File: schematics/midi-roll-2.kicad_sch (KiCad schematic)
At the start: 21 parts, among them M1 Stepper_Motor_unipolar_5pin, SW1 SW_Push_SPDT, SW10 SW_Push_SPDT, SW11 SW_Push_SPDT, SW12 SW_Push_SPDT, SW13 SW_Push_SPDT, SW14 SW_Push_SPDT, SW15 SW_Push_SPDT, SW16 SW_Push_SPDT, SW2 SW_Push_SPDT, SW3 SW_Push_SPDT, SW4 SW_Push_SPDT, SW5 SW_Push_SPDT, SW6 SW_Push_SPDT, SW7 SW_Push_SPDT, SW8 SW_Push_SPDT, SW9 SW_Push_SPDT, U1 WeMos_D1_mini, U2 CD4051B, U3 CD4051B, U4 ULN2003A

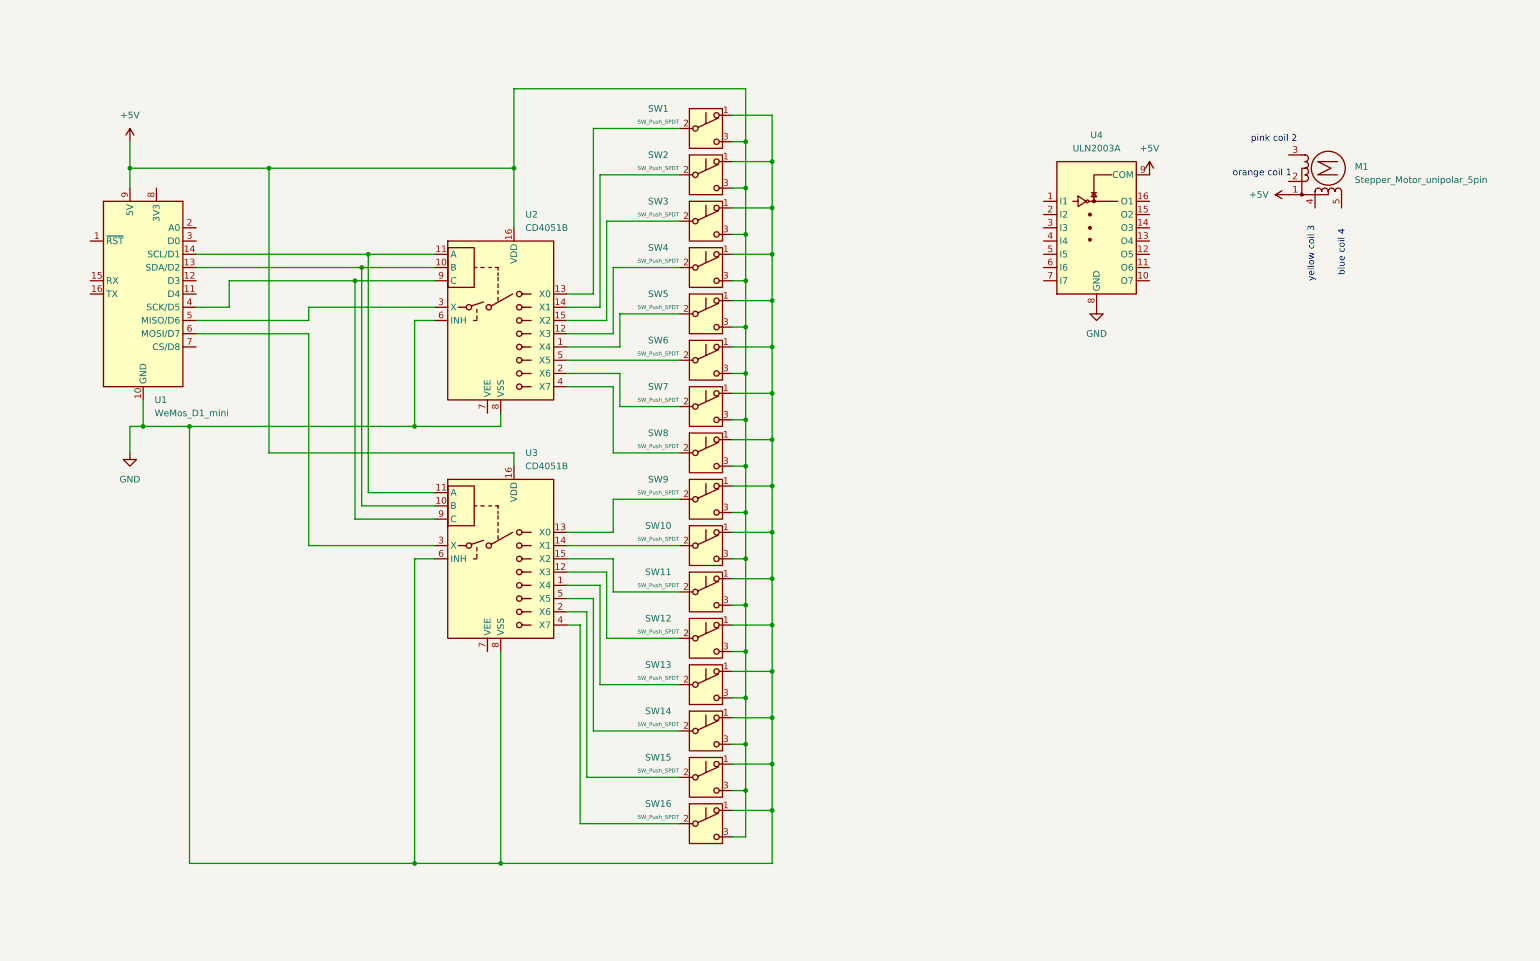
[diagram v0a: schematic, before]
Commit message: updated schematic
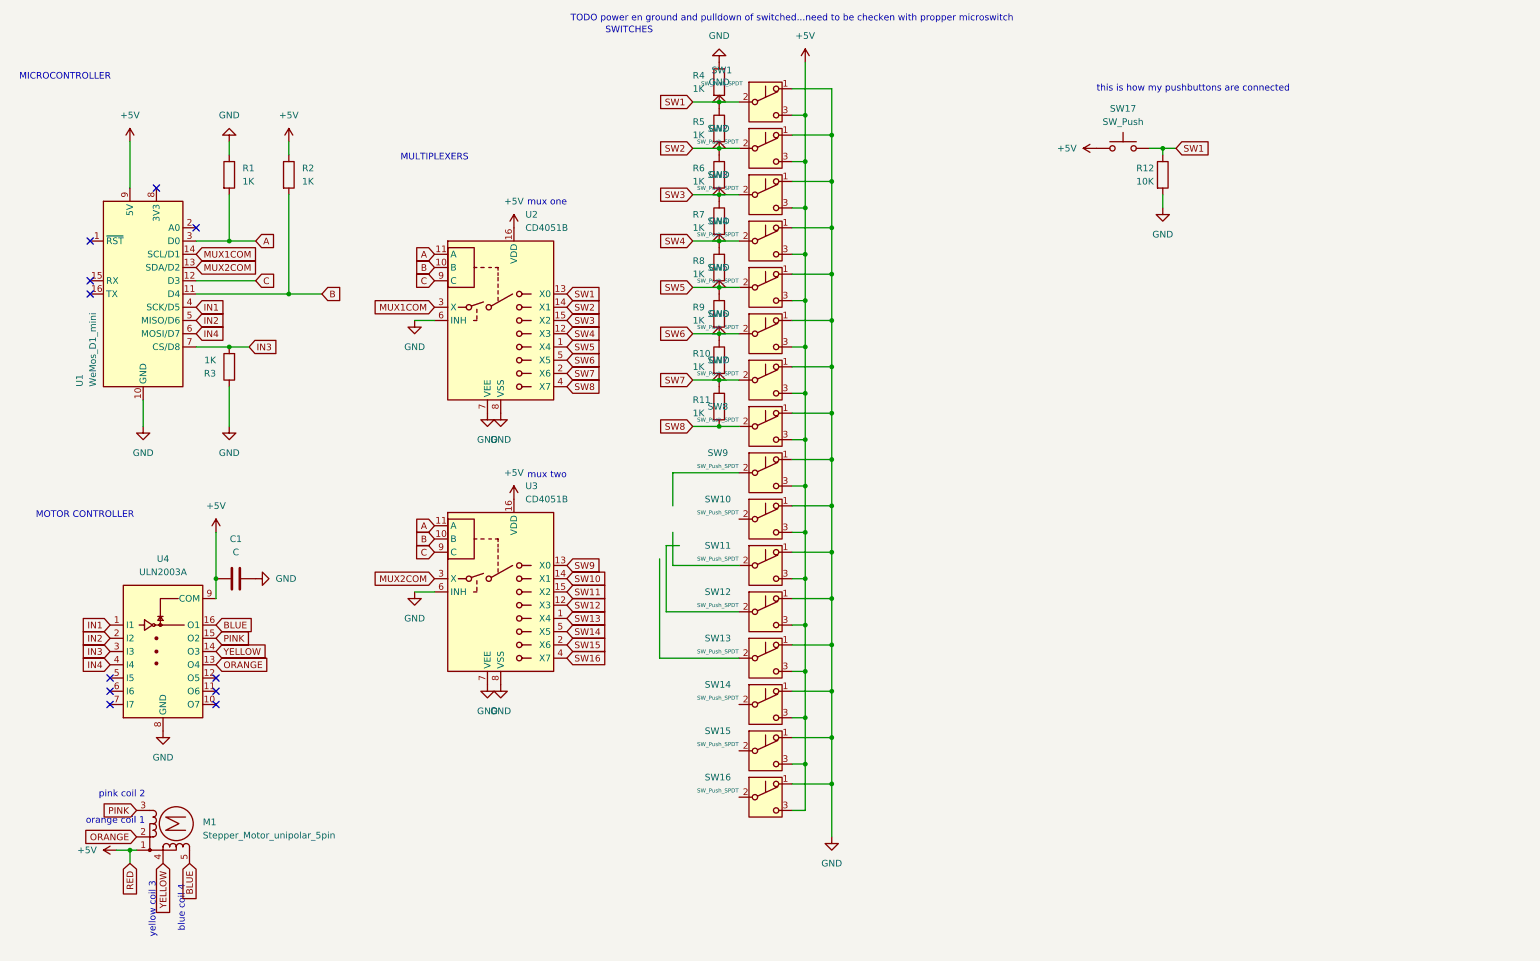
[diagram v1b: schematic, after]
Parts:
- added C1: C, symbol Device:C
- added R1, R10, R11, R2, R3, R4, R5, R6, R7, R8, R9: 1K, symbol Device:R
- added R12: 10K, symbol Device:R
- added SW17: SW_Push, symbol Switch:SW_Push
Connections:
- net +5V: now also C1.1, R2.1, SW17.1
- net GND: now also U2.7 (VEE), U3.7 (VEE), C1.2, R1.1, R10.1, R11.1, R12.2, R3.1, R4.1, R5.1, R6.1, R7.1, R8.1, R9.1
- net SW3: now reaches SW3.2 (B), U2.15 (X2)
- net SW3: now also R6.2
- net at SW13.2 (B): no longer U3.1 (X4)
- net B: now reaches U2.10 (B), U3.10 (B)
- net B: now also U1.11 (D4), R2.2; no longer U1.13 (SDA/D2)
- net A: now reaches U2.11 (A), U3.11 (A)
- net A: now also U1.3 (D0), R1.2; no longer U1.14 (SCL/D1)
- net at SW12.2 (B): no longer U3.12 (X3)
- net at SW9.2 (B): no longer U3.13 (X0)
- net at SW10.2 (B): no longer U3.14 (X1)
- net at SW11.2 (B): no longer U3.15 (X2)
- net at SW15.2 (B): no longer U3.2 (X6)
- net IN4: now reaches U1.6 (MOSI/D7)
- net IN4: now also U4.4 (I4); no longer U3.3 (X)
- net at SW16.2 (B): no longer U3.4 (X7)
- net at SW14.2 (B): no longer U3.5 (X5)
- net C: now reaches U2.9 (C), U3.9 (C)
- net C: now also U1.12 (D3); no longer U1.4 (SCK/D5)
- net SW4: now reaches SW4.2 (B), U2.12 (X3)
- net SW4: now also R7.2
- net ORANGE: now reaches M1.2
- net ORANGE: now also U4.13 (O4)
- net PINK: now reaches M1.3 (-)
- net PINK: now also U4.15 (O2)
- net YELLOW: now reaches M1.4
- net YELLOW: now also U4.14 (O3)
- net BLUE: now reaches M1.5
- net BLUE: now also U4.16 (O1)
- net IN1: now reaches U4.1 (I1)
- net IN1: now also U1.4 (SCK/D5)
- net IN2: now reaches U4.2 (I2)
- net IN2: now also U1.5 (MISO/D6)
- net IN3: now reaches U4.3 (I3)
- net IN3: now also U1.7 (CS/D8), R3.2
- net SW7: now reaches SW7.2 (B), U2.2 (X6)
- net SW7: now also R10.2
- net SW2: now reaches SW2.2 (B), U2.14 (X1)
- net SW2: now also R5.2
- net SW5: now reaches SW5.2 (B), U2.1 (X4)
- net SW5: now also R8.2
- net SW8: now reaches SW8.2 (B), U2.4 (X7)
- net SW8: now also R11.2
- net SW1: now reaches SW1.2 (B), U2.13 (X0)
- net SW1: now also R12.1, R4.2, SW17.2
- net MUX1COM: now reaches U2.3 (X)
- net MUX1COM: now also U1.14 (SCL/D1); no longer U1.5 (MISO/D6)
- net SW6: now reaches SW6.2 (B), U2.5 (X5)
- net SW6: now also R9.2
- new net MUX2COM: U1.13 (SDA/D2), U3.3 (X)
- new net SW10: U3.14 (X1)
- new net SW11: U3.15 (X2)
- new net SW12: U3.12 (X3)
- new net SW13: U3.1 (X4)
- new net SW14: U3.5 (X5)
- new net SW15: U3.2 (X6)
- new net SW16: U3.4 (X7)
- new net SW9: U3.13 (X0)
- no-connect marks 0 -> 11
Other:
- note added: "MICROCONTROLLER"
- note added: "MOTOR CONTROLLER"
- note added: "MULTIPLEXERS"
- note added: "SWITCHES"
- note added: "TODO power en ground and pulldown of switched...need to be checken with propper microswitch"
- note added: "mux one"
- note added: "mux two"
- note added: "this is how my pushbuttons are connected"
- moved on the sheet: M1, SW1, SW10, SW11, SW12, SW13, SW14, SW15, SW16, SW2, SW3, SW4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
